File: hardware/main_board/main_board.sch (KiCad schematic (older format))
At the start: 33 parts, among them J1 eConn_02x03_Odd_Even, P1 CONN_01X02, Q1 DMG3415U, SW1 SW_DPDT_x2, U1 MCP73831/2, U2 AP2112, U3 MCP9808, U4 ESP-WROOM-32D, U5 MMA8451Q

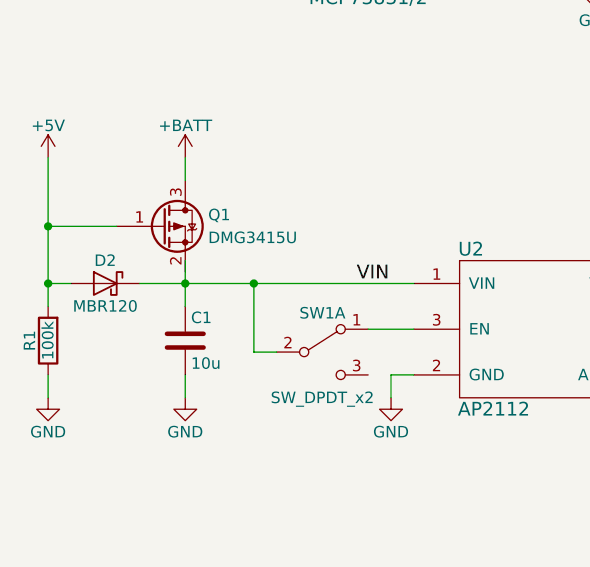
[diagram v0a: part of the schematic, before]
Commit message: Working on component placement
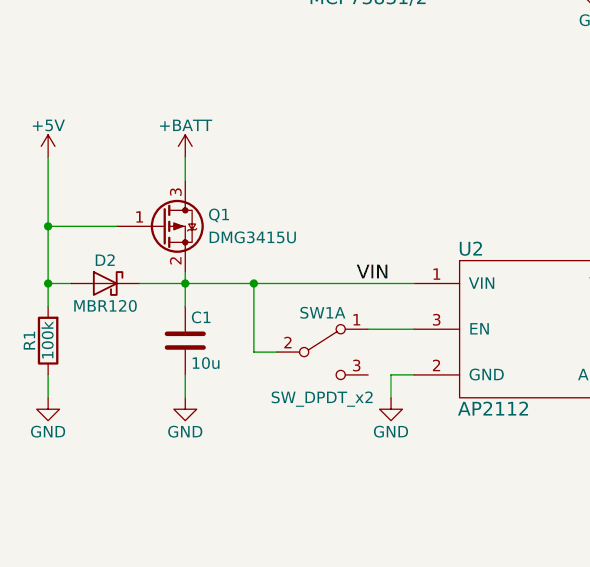
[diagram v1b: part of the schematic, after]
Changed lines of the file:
@@
 Connection ~ 8700 4700
-Wire Wire Line
-	1650 3900 1650 4100
 Wire Wire Line
 	3200 6650 3200 6000
@@
 NoConn ~ 6950 2400
 NoConn ~ 6950 2500
+Wire Wire Line
+	1650 3950 1650 4100
 $EndSCHEMATC
